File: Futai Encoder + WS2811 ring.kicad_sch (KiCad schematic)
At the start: 50 parts, among them J1 Conn_02x05_Top_Bottom, SW1 RotaryEncoder_Switch_RGB

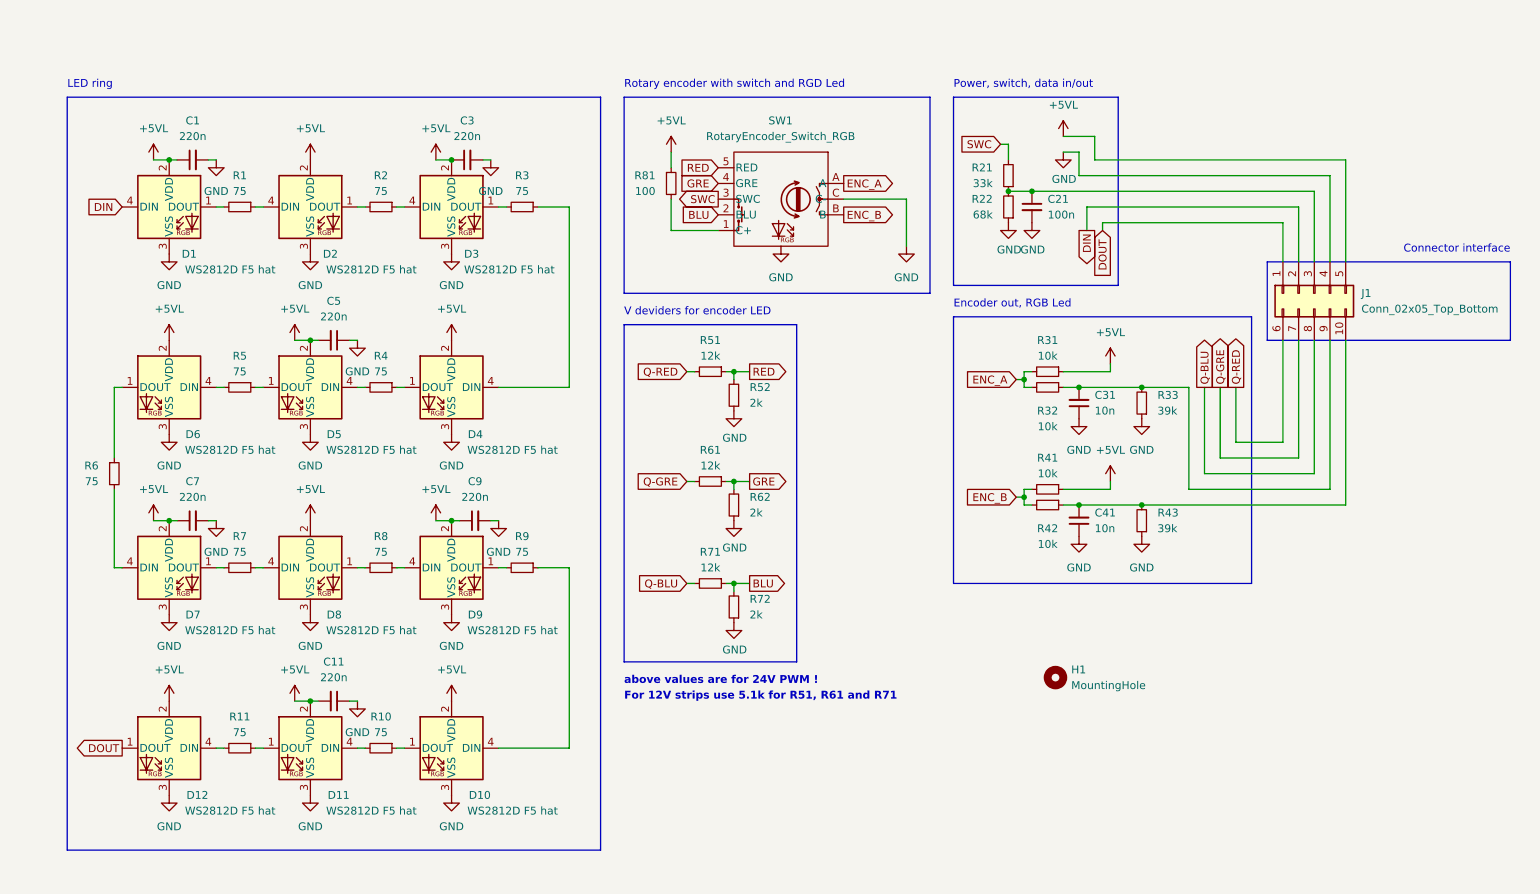
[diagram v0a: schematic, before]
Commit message: brushing up schematic diagram.pdf
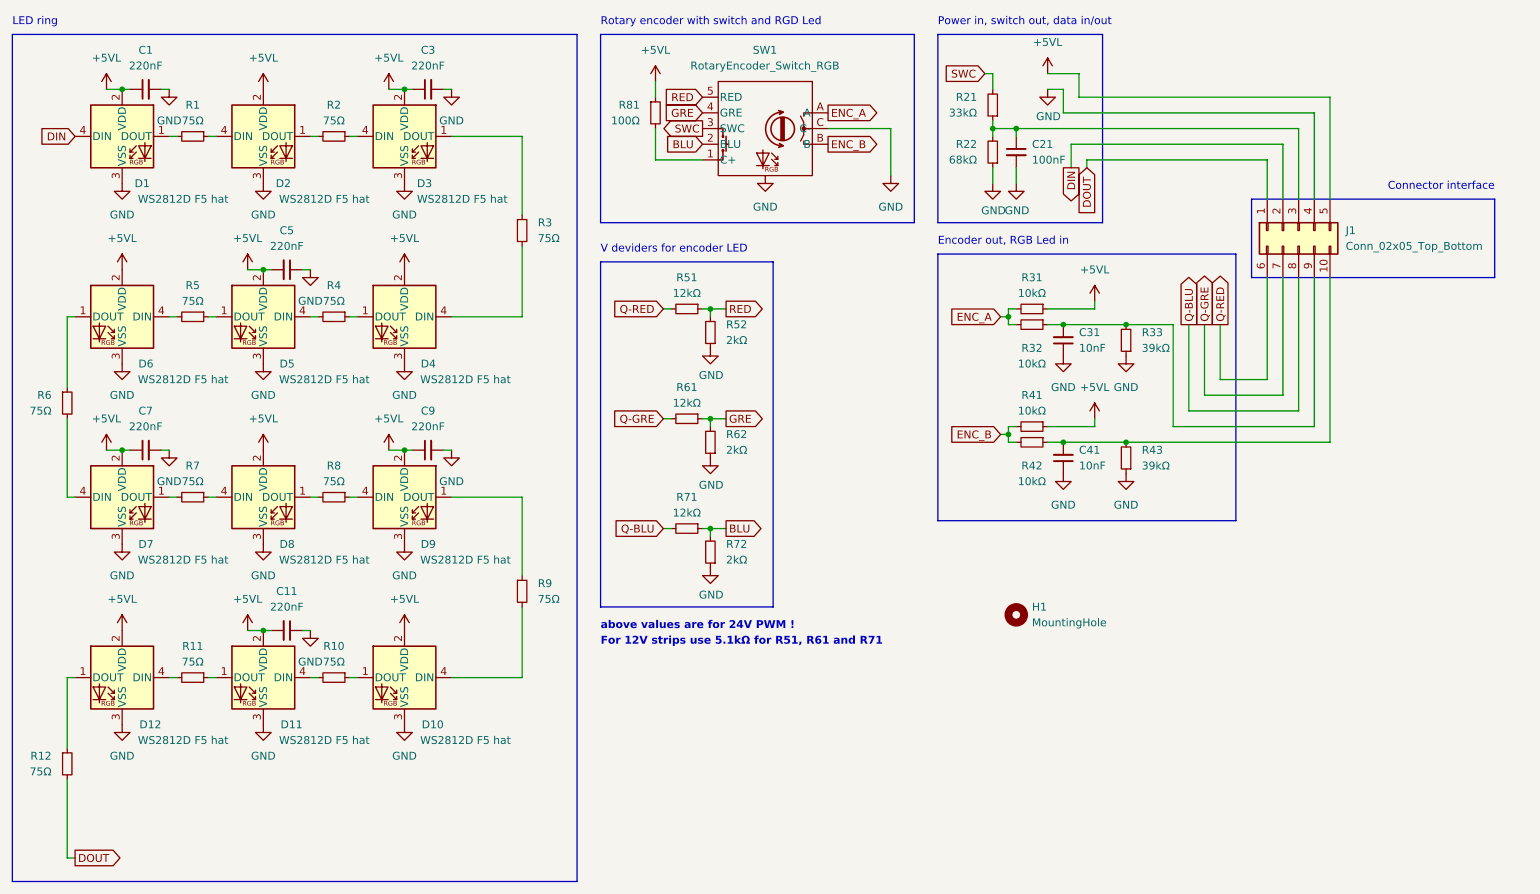
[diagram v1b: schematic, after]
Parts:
- added R12: 75Ω, Resistor_SMD:R_0805_2012Metric, symbol Device:R_Small
- C1, C11, C3, C5, C7, C9: value 220n -> 220nF
- C21: value 100n -> 100nF
- C31, C41: value 10n -> 10nF
- R1, R10, R11, R2, R3, R4, R5, R6, R7, R8, R9: value 75 -> 75Ω
- R21: value 33k -> 33kΩ
- R22: value 68k -> 68kΩ
- R31, R32, R41, R42: value 10k -> 10kΩ
- R33, R43: value 39k -> 39kΩ
- R51, R61, R71: value 12k -> 12kΩ
- R52, R62, R72: value 2k -> 2kΩ
- R81: value 100 -> 100Ω
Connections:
- net DOUT: now also R12.2; no longer D12.1 (DOUT)
- net at D9.1 (DOUT): now also R9.1; no longer R9.2
- net at D10.4 (DIN): now also R9.2; no longer R9.1
- net at D3.1 (DOUT): now also R3.1; no longer R3.2
- net at D4.4 (DIN): now also R3.2; no longer R3.1
- new net: D12.1 (DOUT), R12.1
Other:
- note added: "Encoder out, RGB Led in"
- note added: "For 12V strips use 5.1kΩ for R51, R61 and R71"
- note added: "Power in, switch out, data in/out"
- note removed: "Encoder out, RGB Led"
- note removed: "For 12V strips use 5.1k for R51, R61 and R71"
- note removed: "Power, switch, data in/out"
- moved on the sheet: C1, C11, C21, C3, C31, C41, C5, C7, C9, D1, D10, D11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
